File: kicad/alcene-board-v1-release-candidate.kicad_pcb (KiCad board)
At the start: 2 copper layers, 107 x 87 mm, 16 parts, among them J1 ESP32-S3-DevKitC-1_J1, J2 USB-C Input, J3 ESP32-S3-DevKitC-1_J3, J4 ILI9341_TFT_14pin, J5 Male Pin Header 1x18 - J1 Sig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, J6 Male Pin Header 1x18 - J3 Sig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, J7 Male Pin Header 2x4 - GND, J8 Male Pin Header 2x4 - 3V3, J9 Male Pin Header 2x4 - VIN 5V, SW1 ESP32-S3 Reset (NO momentary)

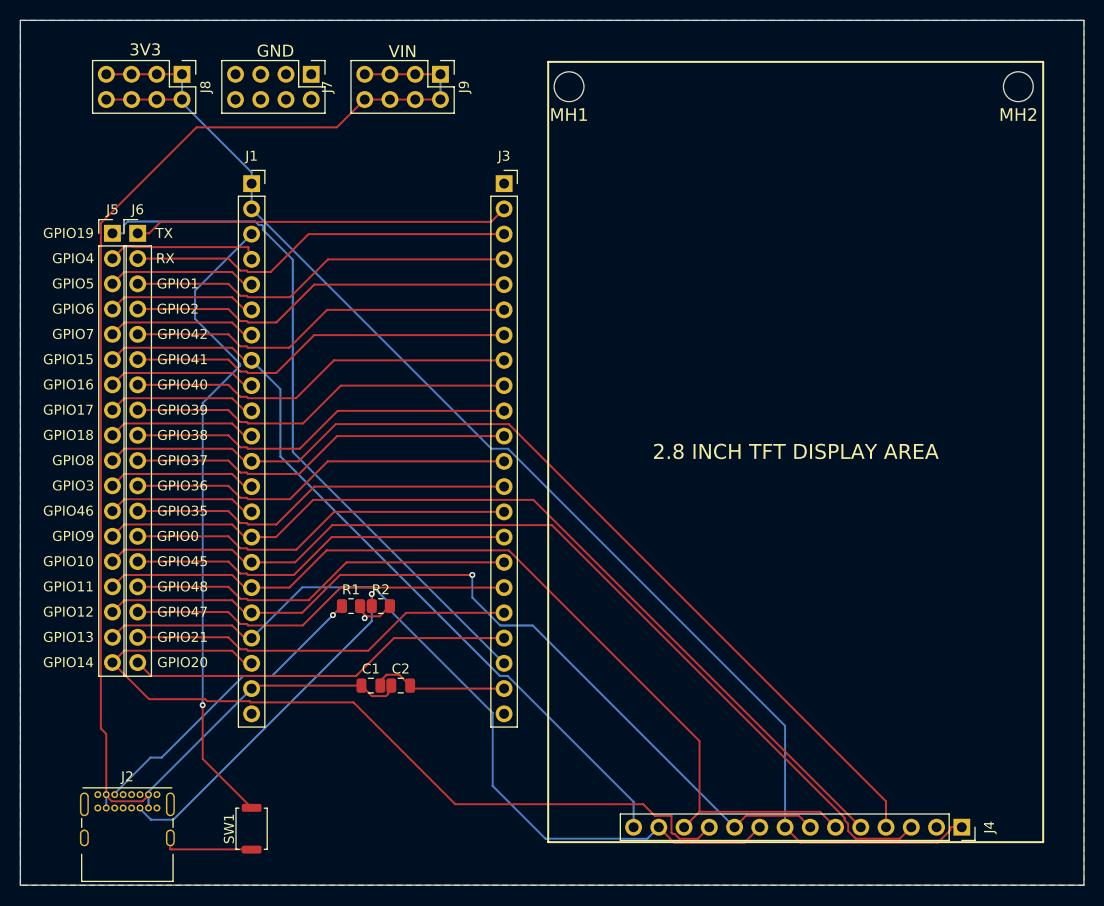
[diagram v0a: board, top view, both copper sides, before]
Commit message: board: rf1
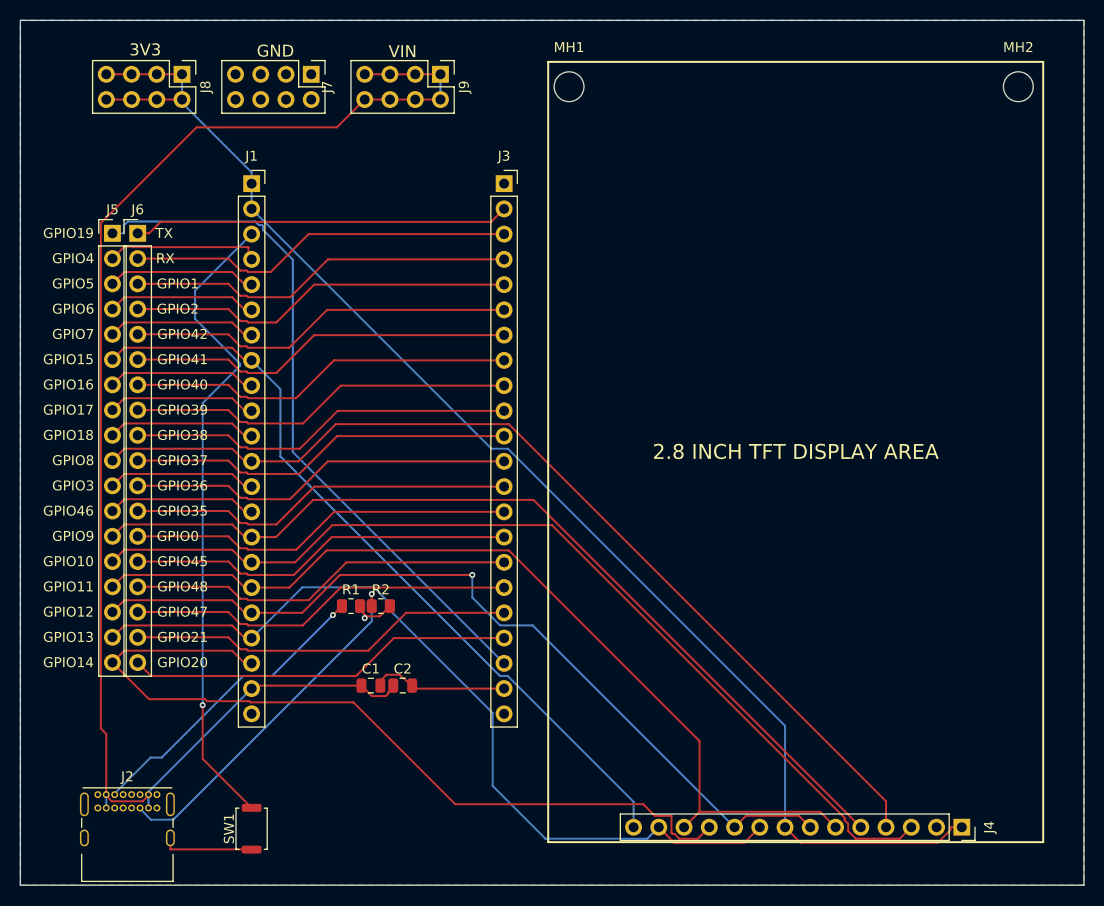
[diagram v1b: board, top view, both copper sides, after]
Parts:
- moved C2 0.20 mm to (72.2, 99.0)
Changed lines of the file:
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@@
 	(footprint "Capacitor_SMD:C_0805_2012Metric"
 		(layer "F.Cu")
-		(at 72 99)
+		(at 72.2 99)
 		(descr "Capacitor SMD 0805 (2012 Metric), square (rectangular) end terminal, IPC-7351 nominal, (Body size source: IPC-SM-782 page 76, https://www.pcb-3d.com/wordpress/wp-content/uploads/ipc-sm-782a_amendment_1_and_2.pdf, https://docs.google.com/spreadsheets/d/1BsfQQcO9C6DZCsRaXUlFlo91Tg2WpOkGARC1WS5S8t0/edit?usp=sharing)")
 		(tags "capacitor")
@@
 			(at 0 45.56 0)
 			(layer "F.Fab")
+			(hide yes)
 			(effects
 				(font
@@
 		)
 	)
+	(footprint "MountingHole:MountingHole_3mm"
+		(layer "F.Cu")
+		(at 88.935715 38.75)
+		(descr "Mounting Hole 3mm, no annular, generated by kicad-footprint-generator mountinghole.py")
+		(tags "mountinghole")
+		(property "Reference" "MH1"
+			(at 0 -3.95 0)
+			(layer "F.SilkS")
+			(effects
+				(font
+					(size 1 1)
+					(thickness 0.15)
+				)
+			)
+		)
+		(property "Value" "MountingHole_3mm"
+			(at 0 3.95 0)
+			(layer "F.Fab")
+			(effects
+				(font
+					(size 1 1)
+					(thickness 0.15)
+				)
+			)
+		)
+		(property "Datasheet" ""
+			(at 0 0 0)
+			(layer "F.Fab")
+			(hide yes)
+			(effects
+				(font
+					(size 1.27 1.27)
+				)
+			)
+		)
+		(property "Description" ""
+			(at 0 0 0)
+			(layer "F.Fab")
+			(hide yes)
+			(effects
+				(font
+					(size 1.27 1.27)
+				)
+			)
+		)
+		(property "KiLib_Generator" "mounting_hardware/mounting_hole"
+			(at 0 0 0)
+			(layer "F.SilkS")
+			(hide yes)
+			(effects
+				(font
+					(size 1 1)
+					(thickness 0.15)
+				)
+			)
+		)
+		(attr exclude_from_pos_files exclude_from_bom)
+		(duplicate_pad_numbers_are_jumpers no)
+		(fp_circle
+			(center 0 0)
+			(end 3 0)
+			(stroke
+				(width 0.15)
+				(type solid)
+			)
+			(fill no)
+			(layer "Cmts.User")
+		)
+		(fp_circle
+			(center 0 0)
+			(end 3.25 0)
+			(stroke
+				(width 0.05)
+				(type solid)
+			)
+			(fill no)
+			(layer "F.CrtYd")
+		)
+		(fp_text user "${REFERENCE}"
+			(at 0 0 0)
+			(layer "F.Fab")
+			(effects
+				(font
+					(size 1 1)
+					(thickness 0.15)
+				)
+			)
+		)
+		(pad "" np_thru_hole circle
+			(at 0 0)
+			(size 3 3)
+			(drill 3)
+			(layers "*.Cu" "*.Mask")
+		)
+		(embedded_fonts no)
+	)
 	(footprint "Button_Switch_SMD:SW_Push_SPST_NO_Alps_SKRK"
 		(layer "F.Cu")
@@
 		)
 	)
+	(footprint "MountingHole:MountingHole_3mm"
+		(layer "F.Cu")
+		(at 134.135715 38.75)
+		(descr "Mounting Hole 3mm, no annular, generated by kicad-footprint-generator mountinghole.py")
+		(tags "mountinghole")
+		(property "Reference" "MH2"
+			(at 0 -3.95 0)
+			(layer "F.SilkS")
+			(effects
+				(font
+					(size 1 1)
+					(thickness 0.15)
+				)
+			)
+		)
+		(property "Value" "MountingHole_3mm"
+			(at 0 3.95 0)
+			(layer "F.Fab")
+			(effects
+				(font
+					(size 1 1)
+					(thickness 0.15)
+				)
+			)
+		)
+		(property "Datasheet" ""
+			(at 0 0 0)
+			(layer "F.Fab")
+			(hide yes)
+			(effects
+				(font
+					(size 1.27 1.27)
+				)
+			)
+		)
+		(property "Description" ""
+			(at 0 0 0)
+			(layer "F.Fab")
+			(hide yes)
+			(effects
+				(font
+					(size 1.27 1.27)
+				)
+			)
+		)
+		(property "KiLib_Generator" "mounting_hardware/mounting_hole"
+			(at 0 0 0)
+			(layer "F.SilkS")
+			(hide yes)
+			(effects
+				(font
+					(size 1 1)
+					(thickness 0.15)
+				)
+			)
+		)
+		(attr exclude_from_pos_files exclude_from_bom)
+		(duplicate_pad_numbers_are_jumpers no)
+		(fp_circle
+			(center 0 0)
+			(end 3 0)
+			(stroke
+				(width 0.15)
+				(type solid)
+			)
+			(fill no)
+			(layer "Cmts.User")
+		)
+		(fp_circle
+			(center 0 0)
+			(end 3.25 0)
+			(stroke
+				(width 0.05)
+				(type solid)
+			)
+			(fill no)
+			(layer "F.CrtYd")
+		)
+		(fp_text user "${REFERENCE}"
+			(at 0 0 0)
+			(layer "F.Fab")
+			(effects
+				(font
+					(size 1 1)
+					(thickness 0.15)
+				)
+			)
+		)
+		(pad "" np_thru_hole circle
+			(at 0 0)
+			(size 3 3)
+			(drill 3)
+			(layers "*.Cu" "*.Mask")
+		)
+		(embedded_fonts no)
+	)
 	(footprint "Connector_USB:USB_C_Receptacle_GCT_USB4085"
 		(layer "F.Cu")
@@
 		)
 	)
-	(footprint "MountingHole:MountingHole_3mm"
-		(layer "F.Cu")
-		(at 134.135715 38.75)
-		(property "Reference" "MH2"
-			(at 0.014285 2.85 0)
-			(layer "F.SilkS")
-			(effects
-				(font
-					(size 1.27 1.27)
-				)
-			)
-		)
-		(property "Value" "MountingHole_3mm"
-			(at 0 0 0)
-			(layer "F.Fab")
-			(effects
-				(font
-					(size 1.27 1.27)
-				)
-			)
-		)
-		(property "Datasheet" ""
-			(at 0 0 0)
-			(layer "F.Fab")
-			(hide yes)
-			(effects
-				(font
-					(size 1.27 1.27)
-				)
-			)
-		)
-		(property "Description" ""
-			(at 0 0 0)
-			(layer "F.Fab")
-			(hide yes)
-			(effects
-				(font
-					(size 1.27 1.27)
-				)
-			)
-		)
-		(duplicate_pad_numbers_are_jumpers no)
-		(pad "" np_thru_hole circle
-			(at 0 0)
-			(size 3 3)
-			(drill 3)
-			(layers "*.Mask")
-		)
-		(embedded_fonts no)
-	)
 	(footprint "Connector_PinSocket_2.54mm:PinSocket_1x22_P2.54mm_Vertical"
 		(layer "F.Cu")
@@
 			(at 1.27 10 270)
 			(layer "F.Fab")
+			(hide yes)
 			(effects
 				(font
@@
 		)
 	)
-	(footprint "MountingHole:MountingHole_3mm"
-		(layer "F.Cu")
-		(at 88.935715 38.75)
-		(property "Reference" "MH1"
-			(at 0 2.85 0)
-			(layer "F.SilkS")
-			(effects
-				(font
-					(size 1.27 1.27)
-				)
-			)
-		)
-		(property "Value" "MountingHole_3mm"
-			(at 0 0 0)
-			(layer "F.Fab")
-			(effects
-				(font
-					(size 1.27 1.27)
-				)
-			)
-		)
-		(property "Datasheet" ""
-			(at 0 0 0)
-			(layer "F.Fab")
-			(hide yes)
-			(effects
-				(font
-					(size 1.27 1.27)
-				)
-			)
-		)
-		(property "Description" ""
-			(at 0 0 0)
-			(layer "F.Fab")
-			(hide yes)
-			(effects
-				(font
-					(size 1.27 1.27)
-				)
-			)
-		)
-		(duplicate_pad_numbers_are_jumpers no)
-		(pad "" np_thru_hole circle
-			(at 0 0)
-			(size 3 3)
-			(drill 3)
-			(layers "*.Mask")
-		)
-		(embedded_fonts no)
-	)
 	(footprint "Capacitor_SMD:C_0805_2012Metric"
 		(layer "F.Cu")
@@
 			(at 0 45.56 0)
 			(layer "F.Fab")
+			(hide yes)
 			(effects
 				(font
@@
 	)
 	(segment
-		(start 71.8589 97.9089)
-		(end 72.95 99)
+		(start 73.25 99.3)
+		(end 73.15 99)
 		(width 0.2)
 		(layer "F.Cu")
@@
 	)
 	(segment
-		(start 73.25 99.3)
-		(end 72.95 99)
-		(width 0.2)
-		(layer "F.Cu")
-		(net "GND")
-	)
-	(segment
 		(start 48.825 115.4779)
 		(end 56.9779 115.4779)
@@
 	)
 	(segment
+		(start 71.8589 97.9089)
+		(end 73.15 99)
+		(width 0.2)
+		(layer "F.Cu")
+		(net "GND")
+	)
+	(segment
 		(start 48.825 114.3262)
 		(end 48.825 115.4779)
@@
 	)
 	(segment
+		(start 71.25 99.4043)
+		(end 71.25 99)
+		(width 0.2)
+		(layer "F.Cu")
+		(net "VIN")
+	)
+	(segment
 		(start 57 99.3)
 		(end 57.3 99)
@@
 	)
 	(segment
-		(start 71.05 99.4043)
-		(end 71.05 99)
+		(start 51.4639 42.8369)
+		(end 65.5831 42.8369)
 		(width 0.2)
 		(layer "F.Cu")
@@
 	)
 	(segment
-		(start 51.4639 42.8369)
-		(end 65.5831 42.8369)
+		(start 70.8285 99.6258)
+		(end 71.25 99.4043)
 		(width 0.2)
 		(layer "F.Cu")
@@
 		(width 0.2)
 		(layer "F.Cu")
-		(net "VIN")
-	)
-	(segment
-		(start 70.8285 99.6258)
-		(end 71.05 99.4043)
-		(width 0.2)
-		(layer "F.Cu")
